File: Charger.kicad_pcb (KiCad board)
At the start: 2 copper layers, 67.3 x 30.6 mm, 12 parts, among them J1 Input, J2 USB-A-S-X-X-SM2, U1 LT1085-5.0

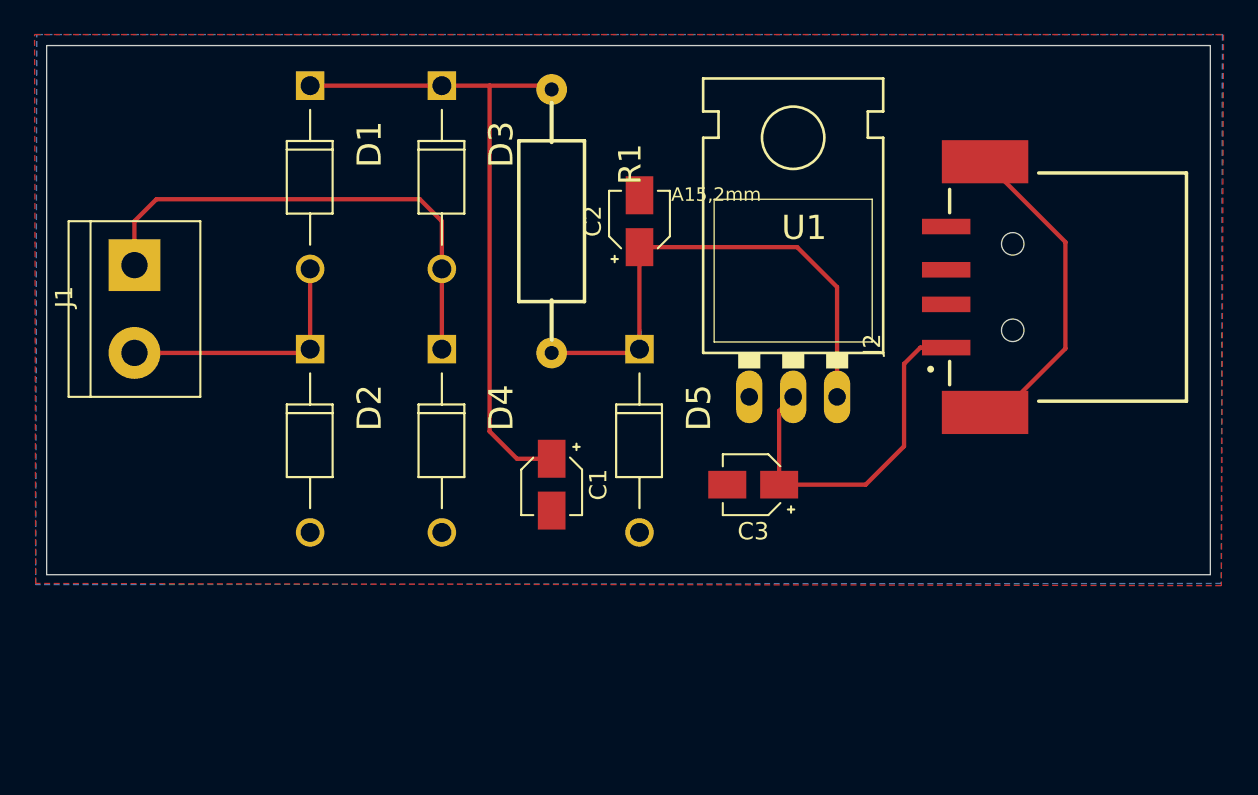
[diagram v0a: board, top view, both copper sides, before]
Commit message: updates schematics
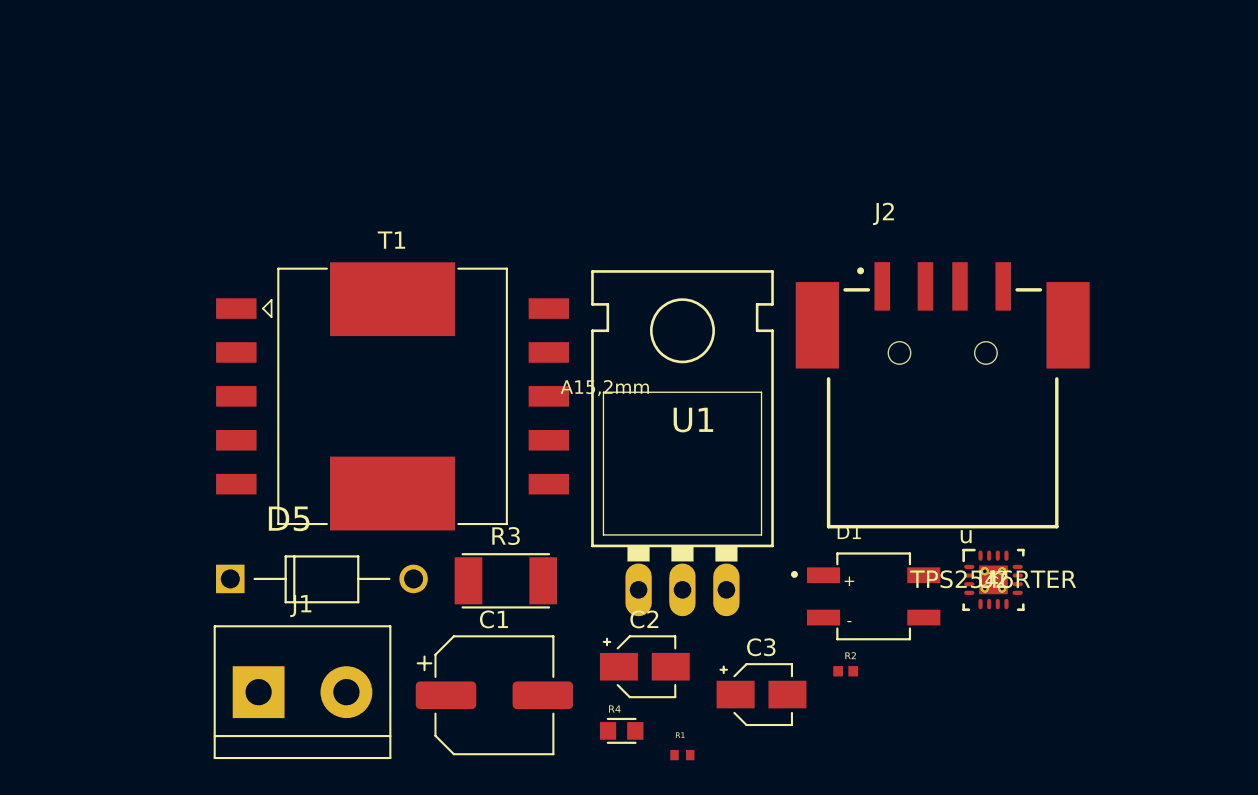
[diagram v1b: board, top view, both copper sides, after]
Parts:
- removed D2, D3, D4: 1N4005, Diode_1n4005:DIOAD1060W80L410D260
- added R2: 100k, R100k:RESC1005X40N, F.Cu at (474.2, 1073.8)
- added R3: 80.6k, R806:RESC5025X70N, F.Cu at (454.6, 1068.6)
- added R4: 16.9k, R169:RESC1608X50N, F.Cu at (461.3, 1077.2)
- added T1: Transformer_12P_1S, Transformer_SMD:Transformer_Coilcraft_CST2010, F.Cu at (448.0, 1057.9)
- added U2: TPS2546RTER, footprints:TPS2546RTER, F.Cu at (482.8, 1068.5)
- C1: value 1m -> 4.7m; footprint Capacitor_SMD:CP_Elec_3x5.3 -> Capacitor_SMD:CP_Elec_6.3x9.9
- D1: value 1N4005 -> D_Bridge_+-AA; footprint Diode_1n4005:DIOAD1060W80L410D260 -> rectifier:SOIC245P670X270-4N
- R1: footprint resist_20:EXC-ELSA39 -> R20:RESC1005X35N
- moved D1 40.6 mm to (475.8, 1069.5), turned to 0 degrees
- moved R1 31.8 mm to (464.8, 1078.6), turned to 0 degrees
- moved C2 25.8 mm to (462.6, 1073.5), turned to 0 degrees
- moved J1 25.7 mm to (440.3, 1075.0), turned to 0 degrees
- moved D5 20.0 mm to (443.9, 1068.4), turned to 0 degrees
- moved U1 12.9 mm to (464.8, 1065.3)
- moved C1 12.6 mm to (453.9, 1075.2), turned to 0 degrees
- moved C3 12.1 mm to (469.3, 1075.1), turned to 0 degrees
- moved J2 5.56 mm to (479.8, 1055.4), turned to 0 degrees
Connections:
- C3 pad 1: Vout -> Vint
- D1 pad 2: - -> gnd
- J1 pad 1: + -> AC1
- J1 pad 2: - -> AC2
- U1 pad 2: Vout -> Vint
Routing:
- net Net-(C1-Pad1): track 38.3 -> 0.00 mm
- net Net-(C2-Pad1): track 30.9 -> 0.00 mm
- net +: track 28.8 -> 0.00 mm
- net Vout: track 21.2 -> 0.00 mm
- net Net-(J2-PadS1): track 19.1 -> 0.00 mm
- net -: track 14.9 -> 0.00 mm
- removed copper zone on B.Cu, net (none)
- removed copper zone on F.Cu, net gnd
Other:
- board outline removed
- board text removed: "1N4005"
- board text removed: "20 ohm"
- board text removed: "BZX85C10"
- board text removed: "LT1085-5.0"
- board text removed: "USB"
- board text removed: "input"
